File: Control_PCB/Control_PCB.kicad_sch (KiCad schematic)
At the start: 3 parts, among them J1 Minifit 2x3, J2 Conn_01x09, J3 Conn_01x05

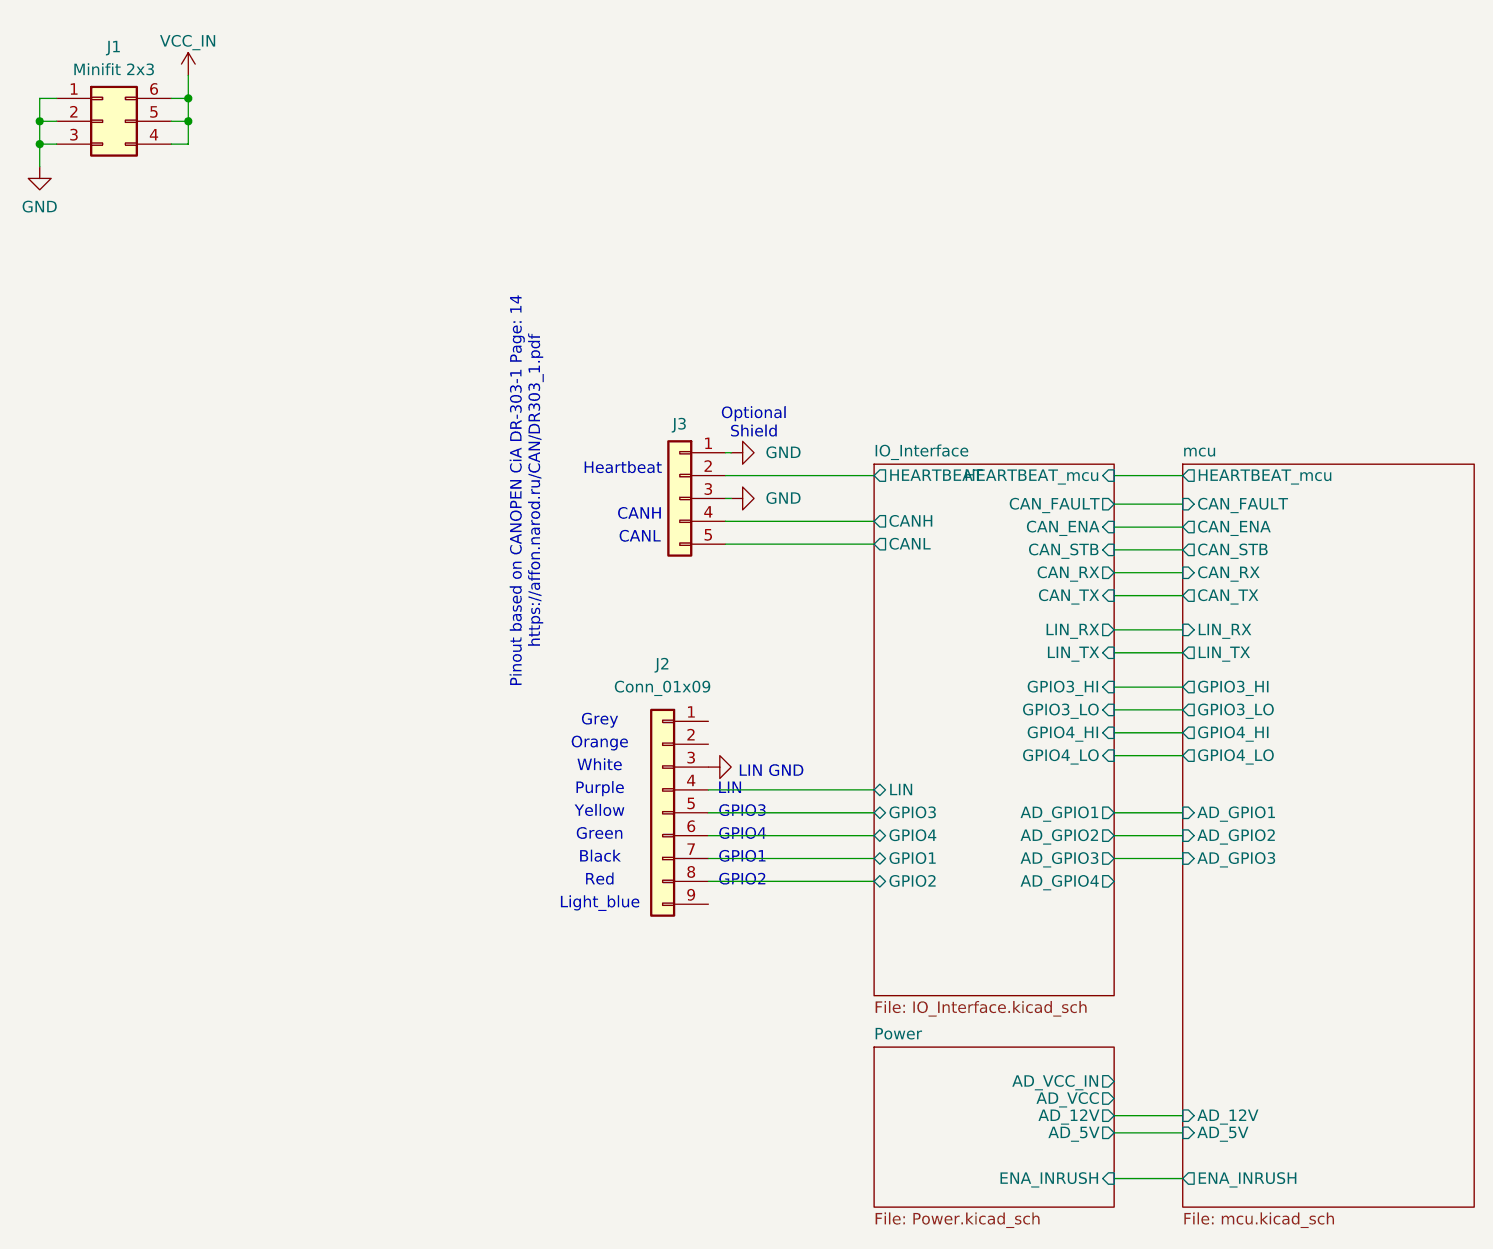
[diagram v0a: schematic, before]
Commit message: 15-10-2026
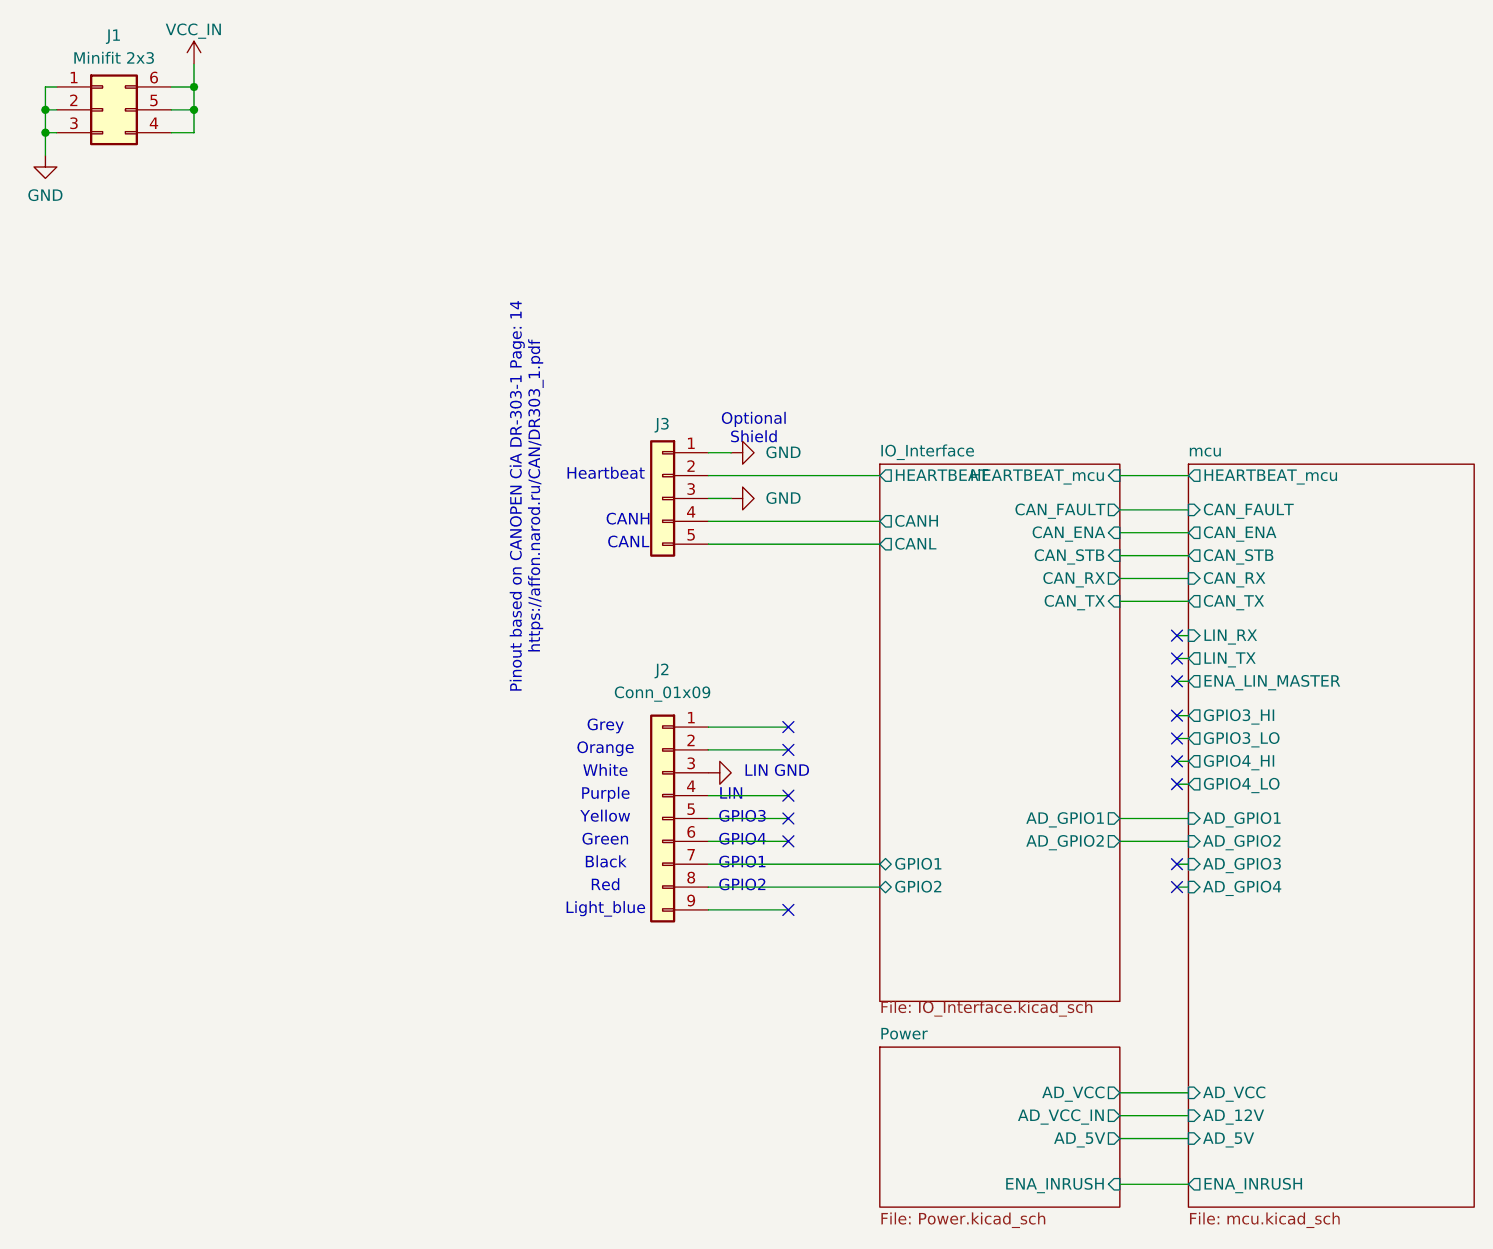
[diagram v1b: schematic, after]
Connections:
- net IO_Interface/GPIO3: no longer names the net of J2.5 (Pin_5)
- net IO_Interface/GPIO4: no longer names the net of J2.6 (Pin_6)
- net IO_Interface/LIN: no longer names the net of J2.4 (Pin_4)
- no-connect marks 0 -> 15
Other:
- sheet IO_Interface ports: added none; removed AD_GPIO3, AD_GPIO4, GPIO3, GPIO3_HI, GPIO3_LO, GPIO4, GPIO4_HI, GPIO4_LO, LIN, LIN_RX, LIN_TX
- sheet Power ports: added none; removed AD_12V
- sheet mcu ports: added AD_GPIO4, AD_VCC, ENA_LIN_MASTER; removed none
- moved on the sheet: J1, J2, J3
